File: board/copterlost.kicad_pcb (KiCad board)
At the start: 2 copper layers, 27.1 x 22.1 mm, 23 parts, among them J1 5V_Copter, J2 Ground, J3 FC.Beeper-, J4 FC.Beeper+, Q1 MMBT3904, Q2 MMBT3904, Q3 MMBT3904, SW1 SW_Push, U1 ATTINY13-20SSU

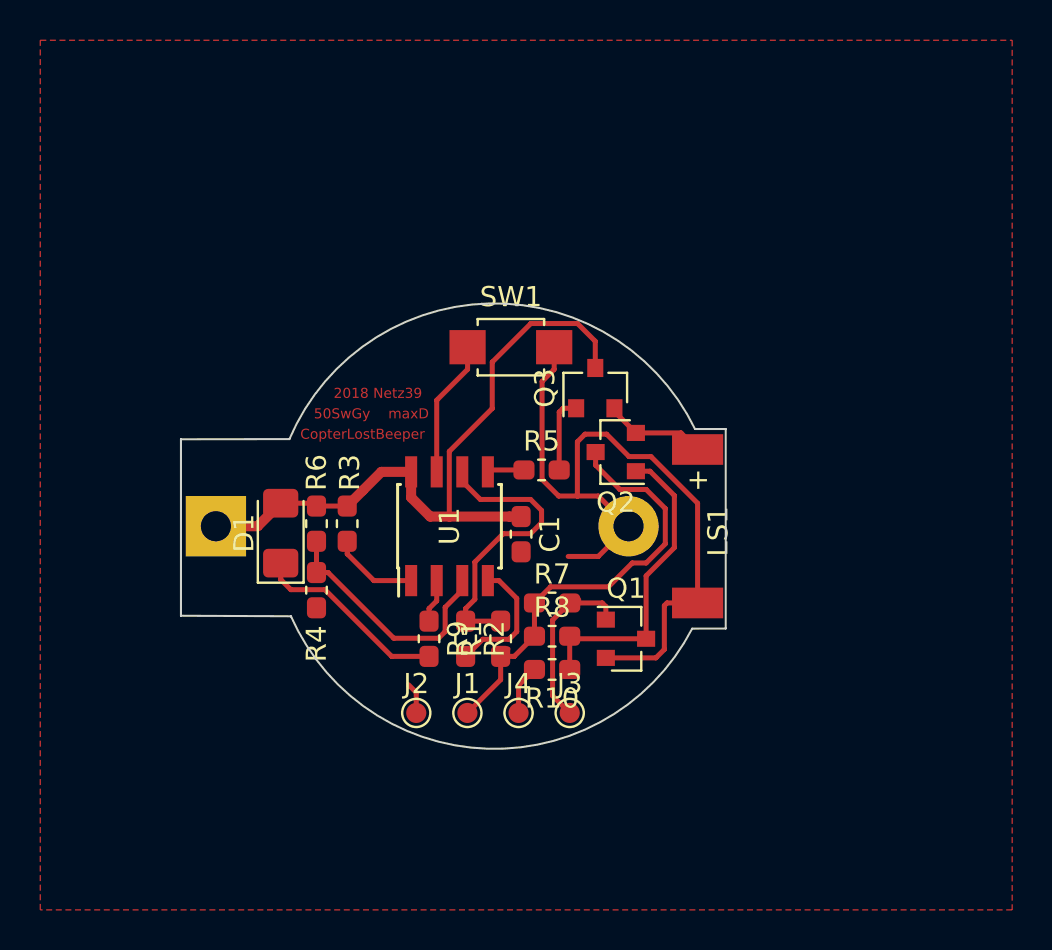
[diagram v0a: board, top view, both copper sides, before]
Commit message: ready to etch
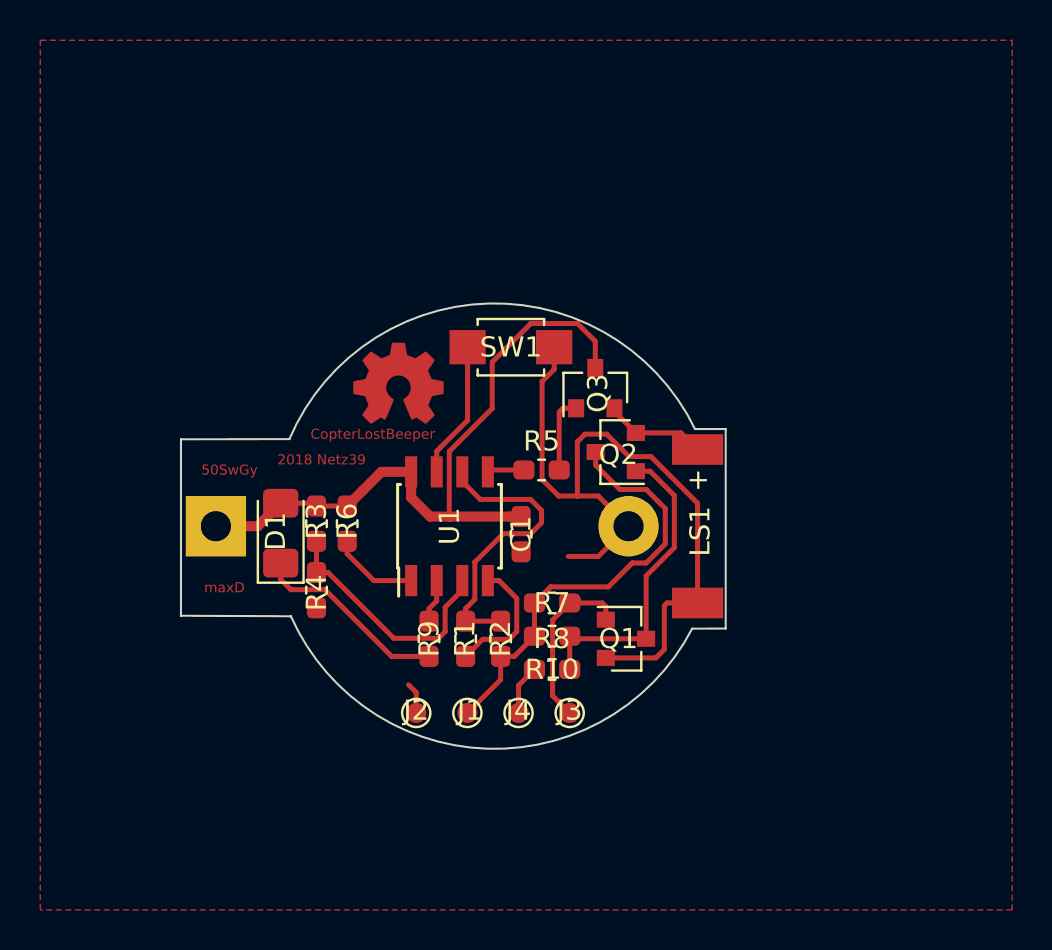
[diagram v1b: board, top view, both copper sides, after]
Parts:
- added REF**: OSHW-Logo_5.7x6mm_Copper, Symbol:OSHW-Logo_5.7x6mm_Copper, F.Cu at (114.3, 71.4)
- R3: value 10k -> 18k

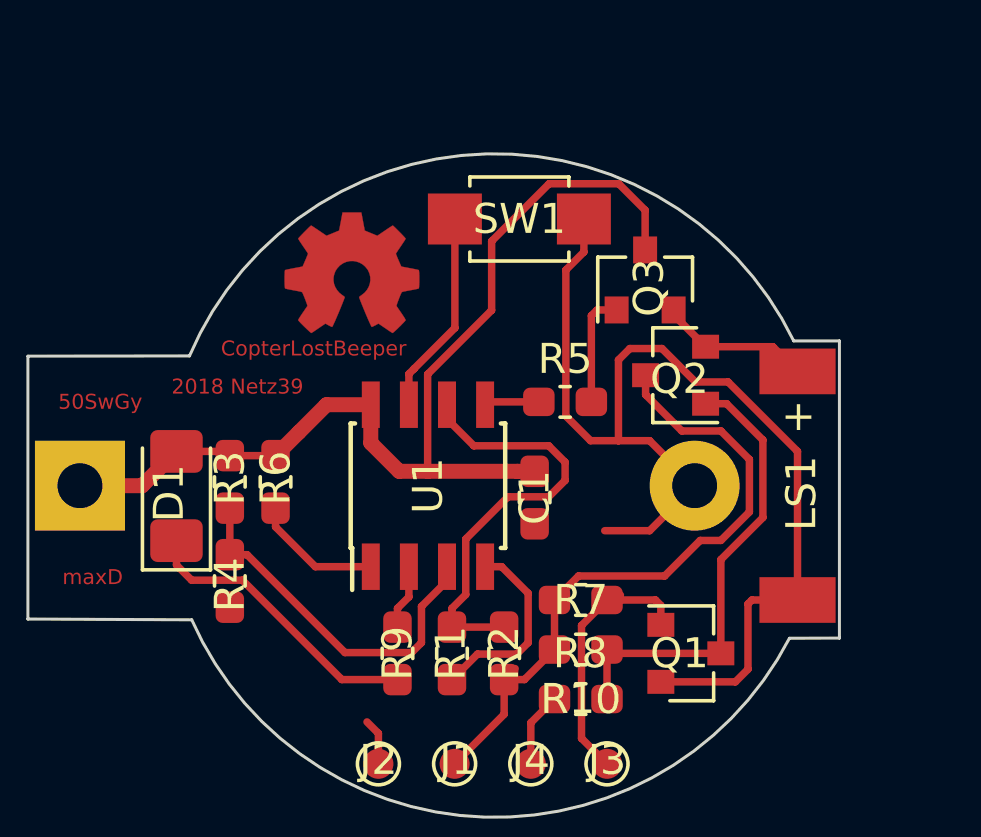
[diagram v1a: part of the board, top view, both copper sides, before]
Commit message: some layout fixes
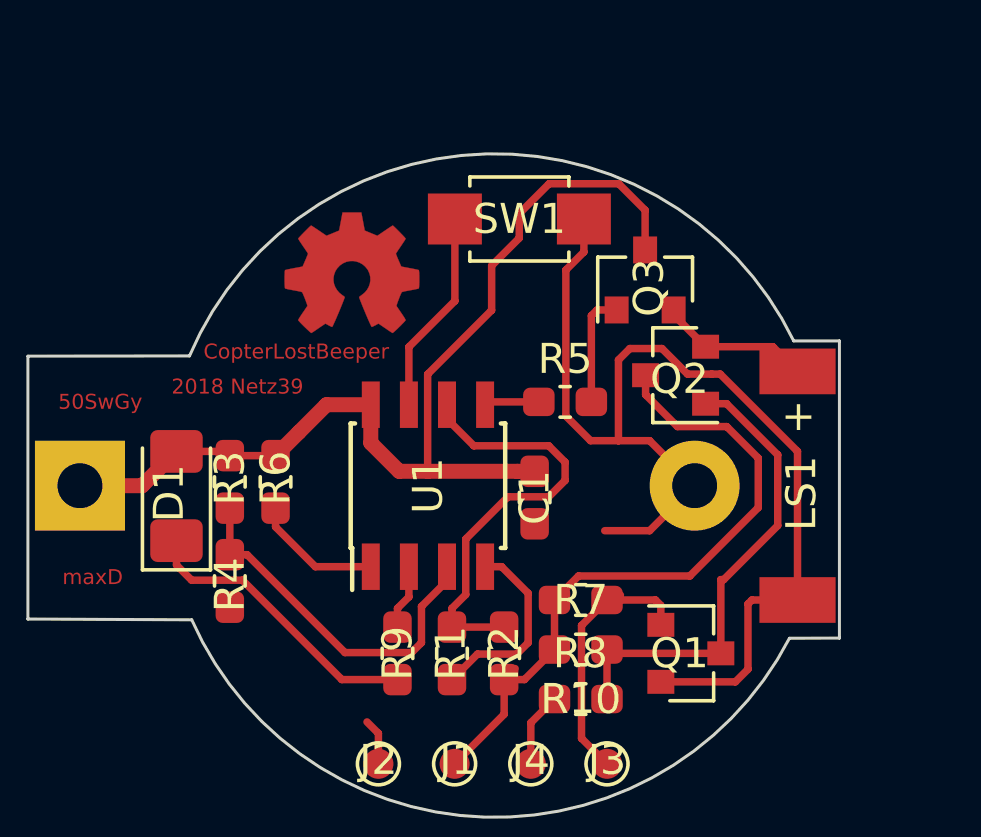
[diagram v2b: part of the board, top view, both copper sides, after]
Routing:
- net +5V: track 22.2 -> 22.8 mm
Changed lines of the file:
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@@
     (visible_elements FFFFFF7F)
     (pcbplotparams
-      (layerselection 0x010fc_ffffffff)
+      (layerselection 0x01000_7fffffff)
       (usegerberextensions false)
       (usegerberattributes false)
@@
       (outputformat 1)
       (mirror false)
-      (drillshape 1)
+      (drillshape 0)
       (scaleselection 1)
-      (outputdirectory ""))
+      (outputdirectory "/home/max/Documents/PlatformIO/Projects/CopterLostBeeper/board/cnc/"))
   )
   (net 0 "")
@@
     (effects (font (size 0.5 0.5) (thickness 0.125)))
   )
-  (gr_text CopterLostBeeper (at 113.03 72.898) (layer F.Cu)
+  (gr_text CopterLostBeeper (at 112.45 73) (layer F.Cu)
     (effects (font (size 0.5 0.5) (thickness 0.125)))
   )
@@
   (segment (start 122.260491 75.970001) (end 123.19 75.970001) (width 0.25) (layer F.Cu) (net 1))
   (segment (start 123.19 75.970001) (end 124.230001 75.970001) (width 0.25) (layer F.Cu) (net 1))
-  (segment (start 125.755001 74.011999) (end 126.843999 74.011999) (width 0.25) (layer F.Cu) (net 1))
-  (segment (start 124.641002 72.898) (end 125.755001 74.011999) (width 0.25) (layer F.Cu) (net 1))
   (segment (start 129.159 76.327) (end 129.159 81.28) (width 0.25) (layer F.Cu) (net 1) (status 20))
-  (segment (start 126.843999 74.011999) (end 129.159 76.327) (width 0.25) (layer F.Cu) (net 1))
   (segment (start 123.19 73.279) (end 123.19 75.970001) (width 0.25) (layer F.Cu) (net 1))
   (segment (start 123.571 72.898) (end 123.19 73.279) (width 0.25) (layer F.Cu) (net 1))
@@
   (segment (start 124.230001 78.969999) (end 125.73 77.47) (width 0.25) (layer F.Cu) (net 1) (status 20))
   (segment (start 122.73259 78.969999) (end 124.230001 78.969999) (width 0.25) (layer F.Cu) (net 1))
+  (segment (start 124.641002 72.898) (end 125.493002 73.75) (width 0.25) (layer F.Cu) (net 1))
+  (segment (start 126.582 73.75) (end 126.3 73.75) (width 0.25) (layer F.Cu) (net 1))
+  (segment (start 129.159 76.327) (end 126.582 73.75) (width 0.25) (layer F.Cu) (net 1))
+  (segment (start 125.493002 73.75) (end 126.3 73.75) (width 0.25) (layer F.Cu) (net 1))
   (segment (start 114.855 74.77) (end 114.935 74.77) (width 0.25) (layer F.Cu) (net 2) (status 30))
   (segment (start 110.095 76.327) (end 110.236 76.468) (width 0.25) (layer F.Cu) (net 2) (status 30))
@@
   (segment (start 114.935 76.045) (end 115.88 76.99) (width 0.5) (layer F.Cu) (net 2))
   (segment (start 114.935 74.77) (end 114.935 76.045) (width 0.5) (layer F.Cu) (net 2) (status 10))
-  (segment (start 116.830001 76.980001) (end 116.84 76.99) (width 0.25) (layer F.Cu) (net 2))
   (segment (start 115.88 76.99) (end 116.84 76.99) (width 0.5) (layer F.Cu) (net 2))
-  (segment (start 123.198001 67.404999) (end 120.877999 67.404999) (width 0.25) (layer F.Cu) (net 2))
-  (segment (start 124.079 68.285998) (end 123.198001 67.404999) (width 0.25) (layer F.Cu) (net 2))
-  (segment (start 120.877999 67.404999) (end 118.963001 69.319997) (width 0.25) (layer F.Cu) (net 2))
-  (segment (start 118.963001 69.319997) (end 118.963001 71.621997) (width 0.25) (layer F.Cu) (net 2))
-  (segment (start 116.830001 73.754997) (end 116.830001 76.980001) (width 0.25) (layer F.Cu) (net 2))
   (segment (start 116.84 76.99) (end 119.821 76.99) (width 0.5) (layer F.Cu) (net 2))
   (segment (start 111.76 76.468) (end 112.536 75.692) (width 0.5) (layer F.Cu) (net 2) (status 10))
-  (segment (start 124.079 69.612) (end 124.079 68.285998) (width 0.25) (layer F.Cu) (net 2))
-  (segment (start 118.963001 71.621997) (end 116.830001 73.754997) (width 0.25) (layer F.Cu) (net 2))
+  (segment (start 124.079 68.285998) (end 124.079 69.612) (width 0.25) (layer F.Cu) (net 2))
+  (segment (start 120.877999 67.404999) (end 123.198001 67.404999) (width 0.25) (layer F.Cu) (net 2))
+  (segment (start 116.84 76.99) (end 116.830001 76.980001) (width 0.25) (layer F.Cu) (net 2))
+  (segment (start 123.198001 67.404999) (end 124.079 68.285998) (width 0.25) (layer F.Cu) (net 2))
+  (segment (start 116.830001 76.980001) (end 116.830001 73.754997) (width 0.25) (layer F.Cu) (net 2))
+  (segment (start 119.882998 68.4) (end 120.877999 67.404999) (width 0.25) (layer F.Cu) (net 2))
+  (segment (start 116.830001 73.754997) (end 118.963001 71.621997) (width 0.25) (layer F.Cu) (net 2))
+  (segment (start 118.963001 71.621997) (end 118.963001 70.136999) (width 0.25) (layer F.Cu) (net 2))
+  (segment (start 118.963001 70.136999) (end 119.882998 69.217002) (width 0.25) (layer F.Cu) (net 2))
+  (segment (start 119.882998 69.217002) (end 119.882998 68.4) (width 0.25) (layer F.Cu) (net 2))
   (segment (start 115.824 83.933) (end 113.96951 83.933) (width 0.25) (layer F.Cu) (net 3) (status 10))
   (segment (start 108.458 80.1145) (end 108.458 79.302) (width 0.25) (layer F.Cu) (net 3) (status 20))
@@
   (segment (start 120.057 83.933) (end 119.38 83.933) (width 0.25) (layer F.Cu) (net 4) (status 20))
   (segment (start 121.059 82.931) (end 120.057 83.933) (width 0.25) (layer F.Cu) (net 4) (status 10))
-  (segment (start 127.555001 78.346001) (end 126.606001 79.295001) (width 0.25) (layer F.Cu) (net 4))
-  (segment (start 125.914989 79.295001) (end 124.73 80.47999) (width 0.25) (layer F.Cu) (net 4))
-  (segment (start 124.73 80.47999) (end 121.85901 80.47999) (width 0.25) (layer F.Cu) (net 4))
-  (segment (start 126.606001 79.295001) (end 125.914989 79.295001) (width 0.25) (layer F.Cu) (net 4))
-  (segment (start 121.85901 80.47999) (end 121.059 81.28) (width 0.25) (layer F.Cu) (net 4) (status 20))
-  (segment (start 124.095 74.437) (end 125.302999 75.644999) (width 0.25) (layer F.Cu) (net 4))
-  (segment (start 126.606001 75.644999) (end 127.555001 76.593999) (width 0.25) (layer F.Cu) (net 4))
-  (segment (start 124.095 73.787) (end 124.095 74.437) (width 0.25) (layer F.Cu) (net 4) (status 10))
-  (segment (start 125.302999 75.644999) (end 126.606001 75.644999) (width 0.25) (layer F.Cu) (net 4))
-  (segment (start 127.555001 76.593999) (end 127.555001 78.346001) (width 0.25) (layer F.Cu) (net 4))
+  (segment (start 121.85901 80.47999) (end 121.059 81.28) (width 0.25) (layer F.Cu) (net 4))
+  (segment (start 124.095 73.787) (end 124.095 74.437) (width 0.25) (layer F.Cu) (net 4))
+  (segment (start 126.8 75.5) (end 127.85 76.55) (width 0.25) (layer F.Cu) (net 4))
+  (segment (start 124.095 74.437) (end 125.158 75.5) (width 0.25) (layer F.Cu) (net 4))
+  (segment (start 125.158 75.5) (end 126.8 75.5) (width 0.25) (layer F.Cu) (net 4))
+  (segment (start 127.85 76.55) (end 127.85 78.2) (width 0.25) (layer F.Cu) (net 4))
+  (segment (start 125.57001 80.47999) (end 121.85901 80.47999) (width 0.25) (layer F.Cu) (net 4))
+  (segment (start 127.85 78.2) (end 125.57001 80.47999) (width 0.25) (layer F.Cu) (net 4))
   (segment (start 123.25601 81.11499) (end 122.955072 81.415928) (width 0.25) (layer F.Cu) (net 5) (status 30))
   (segment (start 123.284411 81.28) (end 122.809 81.28) (width 0.25) (layer F.Cu) (net 5) (status 30))
@@
   (segment (start 122.936 83.058) (end 122.809 82.931) (width 0.25) (layer F.Cu) (net 8) (status 30))
   (segment (start 126.603 83.058) (end 122.936 83.058) (width 0.25) (layer F.Cu) (net 8) (status 30))
-  (segment (start 126.603 79.934413) (end 126.603 83.058) (width 0.25) (layer F.Cu) (net 8) (status 20))
-  (segment (start 128.005012 78.532401) (end 126.603 79.934413) (width 0.25) (layer F.Cu) (net 8))
-  (segment (start 128.005012 75.947012) (end 128.005012 78.532401) (width 0.25) (layer F.Cu) (net 8))
-  (segment (start 126.795 74.737) (end 128.005012 75.947012) (width 0.25) (layer F.Cu) (net 8))
-  (segment (start 126.095 74.737) (end 126.795 74.737) (width 0.25) (layer F.Cu) (net 8) (status 10))
+  (segment (start 128.5 76.442) (end 126.795 74.737) (width 0.25) (layer F.Cu) (net 8))
+  (segment (start 128.5 78.8) (end 128.5 76.442) (width 0.25) (layer F.Cu) (net 8))
+  (segment (start 126.795 74.737) (end 126.095 74.737) (width 0.25) (layer F.Cu) (net 8))
+  (segment (start 126.7 80.6) (end 128.5 78.8) (width 0.25) (layer F.Cu) (net 8))
+  (segment (start 126.603 80.6) (end 126.7 80.6) (width 0.25) (layer F.Cu) (net 8))
+  (segment (start 126.603 83.058) (end 126.603 80.6) (width 0.25) (layer F.Cu) (net 8))
   (segment (start 122.303 74.66) (end 122.287 74.676) (width 0.25) (layer F.Cu) (net 9) (status 30))
   (segment (start 122.479 71.612) (end 123.129 71.612) (width 0.25) (layer F.Cu) (net 9) (status 20))
@@
   (segment (start 116.205 81.177) (end 116.205 80.17) (width 0.25) (layer F.Cu) (net 14) (status 20))
   (segment (start 117.688 68.58) (end 117.738 68.58) (width 0.25) (layer F.Cu) (net 15) (status 30))
-  (segment (start 116.379992 73.568596) (end 117.738 72.210588) (width 0.25) (layer F.Cu) (net 15))
-  (segment (start 117.738 72.210588) (end 117.738 68.58) (width 0.25) (layer F.Cu) (net 15))
-  (segment (start 116.205 73.745) (end 116.379991 73.570009) (width 0.25) (layer F.Cu) (net 15))
-  (segment (start 116.379991 73.570009) (end 116.379992 73.568596) (width 0.25) (layer F.Cu) (net 15))
-  (segment (start 116.205 74.77) (end 116.205 73.745) (width 0.25) (layer F.Cu) (net 15))
+  (segment (start 117.738 68.58) (end 117.738 71.312) (width 0.25) (layer F.Cu) (net 15))
+  (segment (start 116.205 72.845) (end 116.205 74.77) (width 0.25) (layer F.Cu) (net 15))
+  (segment (start 117.738 71.312) (end 116.205 72.845) (width 0.25) (layer F.Cu) (net 15))
   (zone (net 1) (net_name GND) (layer F.Cu) (hatch edge 0.508)
     (connect_pads (clearance 0.508))

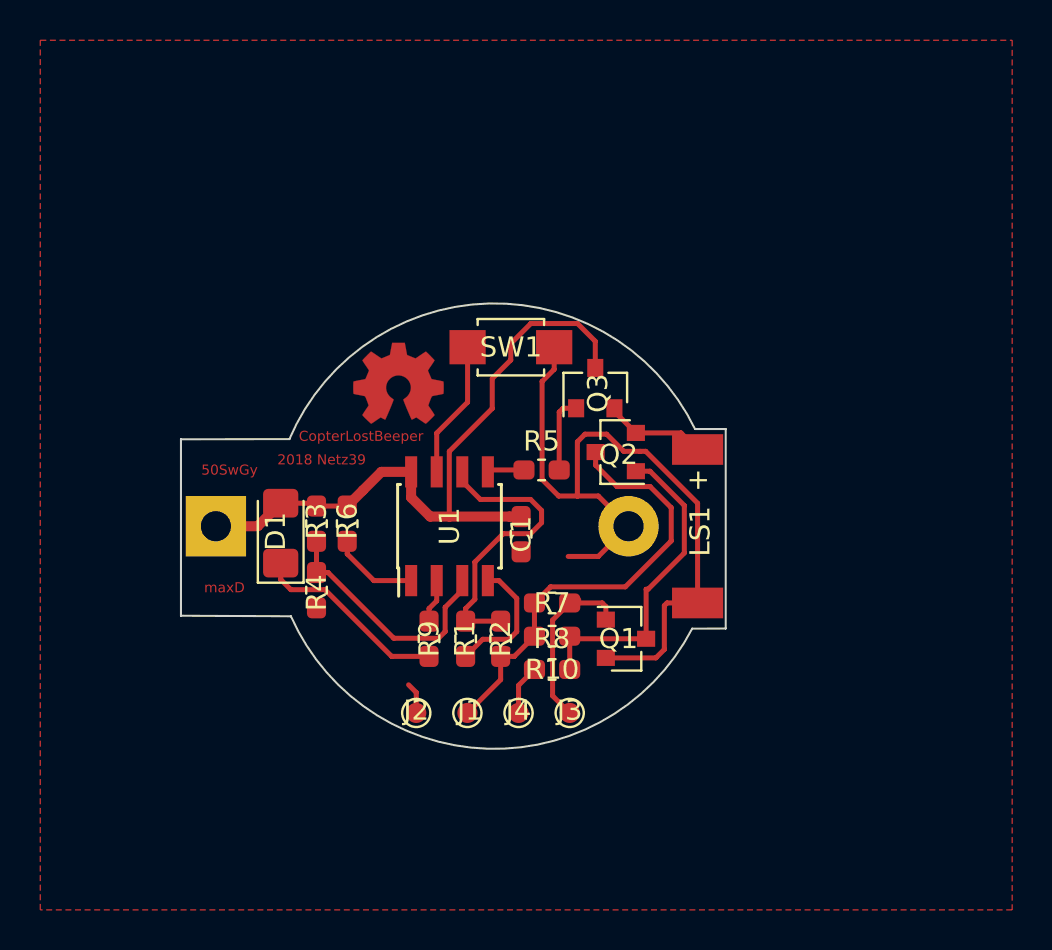
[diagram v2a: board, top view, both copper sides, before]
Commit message: working version
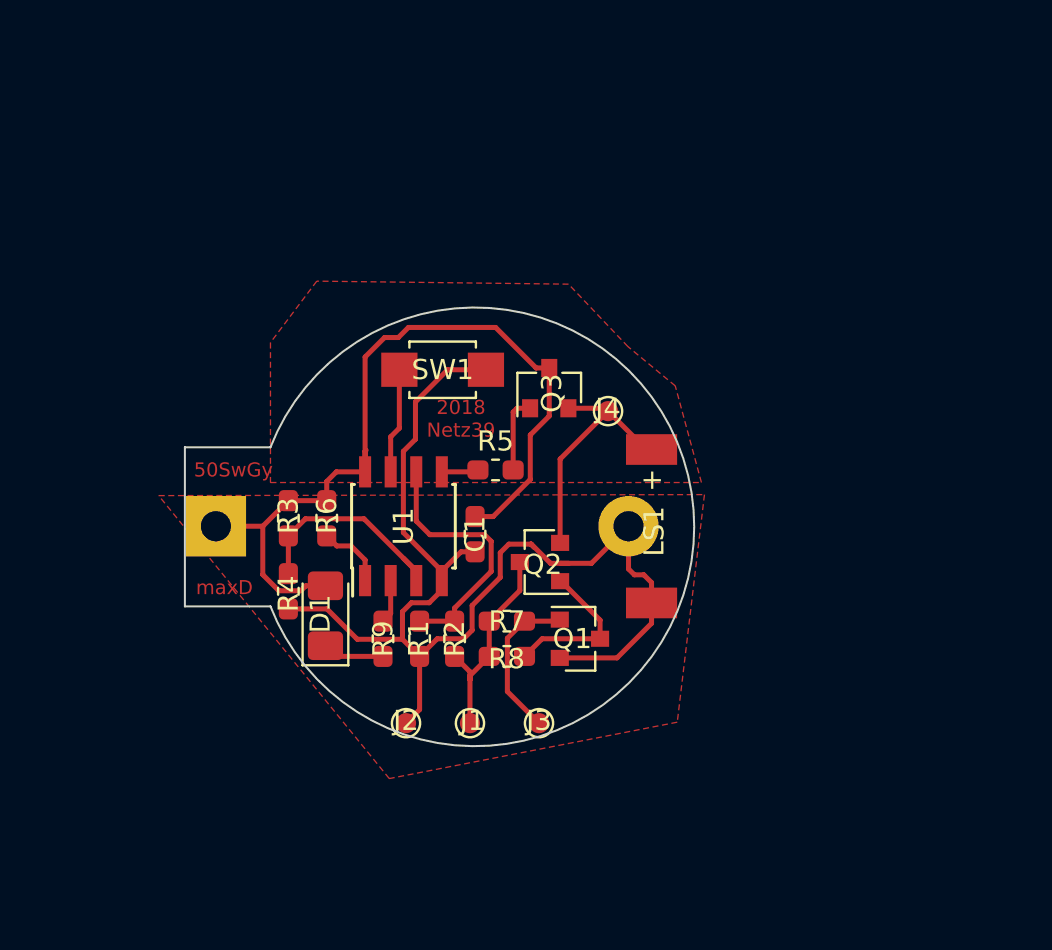
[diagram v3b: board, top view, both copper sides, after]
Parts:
- removed R10: 5k, Resistor_SMD:R_0603_1608Metric_Pad1.05x0.95mm_HandSolder
- removed REF**: OSHW-Logo_5.7x6mm_Copper, Symbol:OSHW-Logo_5.7x6mm_Copper
- R1, R4, R8: value 5k -> 5.1k
- R9: value 50 -> 47
- moved J4 15.6 mm to (124.7, 71.8)
- moved Q2 6.63 mm to (121.3, 79.2)
- moved D1 4.66 mm to (110.7, 81.9)
- moved SW1 3.57 mm to (116.5, 69.7)
- moved R8 2.46 mm to (119.7, 83.9)
- moved R7 2.42 mm to (119.7, 82.2)
- moved C1 2.29 mm to (118.1, 77.9)
- moved Q1 2.29 mm to (123.3, 83.1)
- moved R1 2.29 mm to (117.1, 83.1)
- moved R2 2.29 mm to (115.4, 83.1)
- moved R5 2.29 mm to (119.1, 74.7)
- moved R9 2.29 mm to (113.5, 83.1)
- moved U1 2.29 mm to (114.6, 77.5)
- moved LS1 2.29 mm to (126.9, 77.5)
- moved Q3 2.29 mm to (121.8, 70.6)
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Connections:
- J4 pad 1: Net-(J4-Pad1) -> /Speaker
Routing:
- net +5V: track 22.8 -> 10.5 mm
- net GND: track 45.9 -> 57.8 mm
- net Net-(Q1-Pad3): track 16.4 -> 7.83 mm
- net /Speaker: track 5.07 -> 12.5 mm
- net Net-(D1-Pad1): track 9.76 -> 3.08 mm
- net +BATT: track 37.2 -> 42.3 mm
- net Net-(J4-Pad1): track 2.63 -> 0.00 mm
- net Net-(J3-Pad1): track 9.63 -> 7.85 mm
- net /Button: track 6.87 -> 5.25 mm
- net /Sense: track 14.6 -> 13.0 mm
- net /Batt-Sense: track 12.3 -> 11.0 mm
- net Net-(R6-Pad1): track 4.35 -> 3.42 mm
- added copper zone on F.Cu, net +BATT
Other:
- board size 27.1 x 22.1 mm -> 25.3 x 21.8 mm
- board text removed: "CopterLostBeeper"
